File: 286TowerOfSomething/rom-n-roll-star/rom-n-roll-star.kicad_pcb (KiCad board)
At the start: 2 copper layers, 15 parts, among them J1 Bus_ISA_8bit, SW1 SW_DIP_x08, U1 SST39SF010, U2 74ALS688

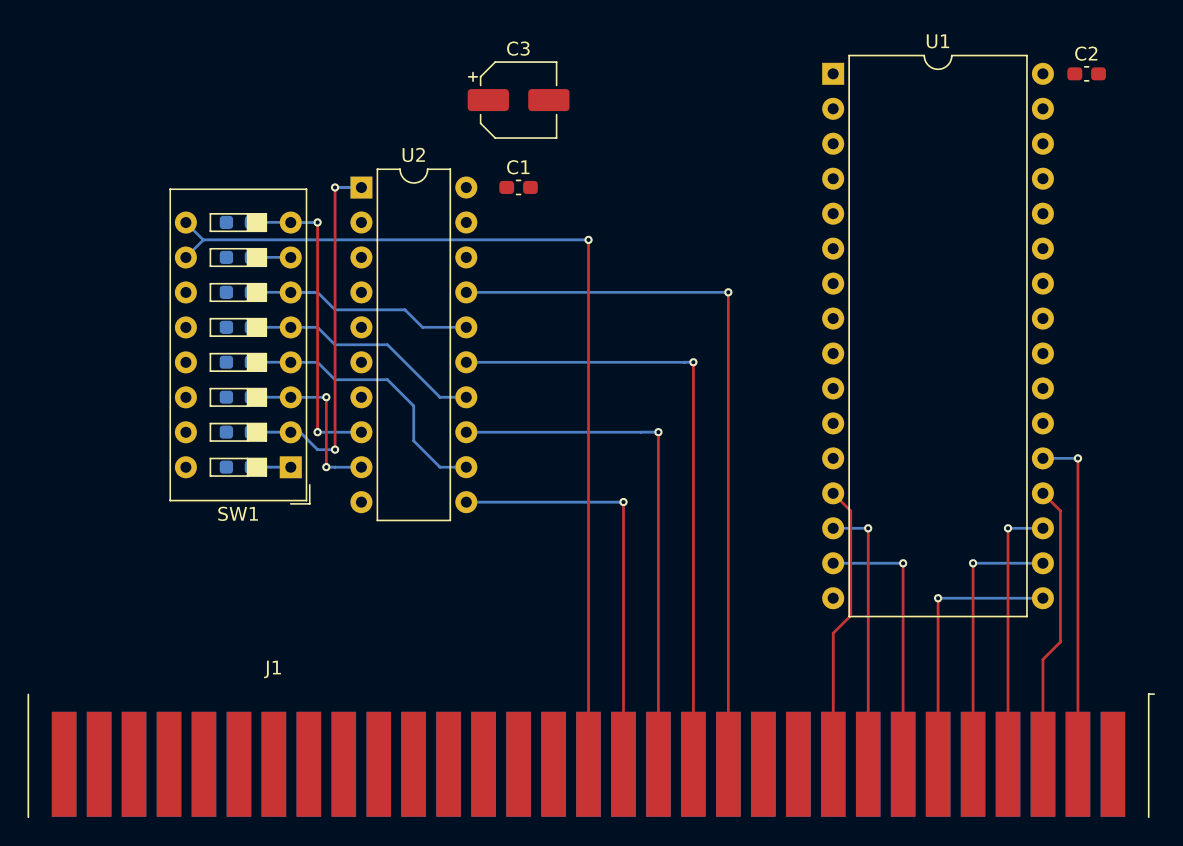
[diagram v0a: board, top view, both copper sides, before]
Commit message: Finished routing?
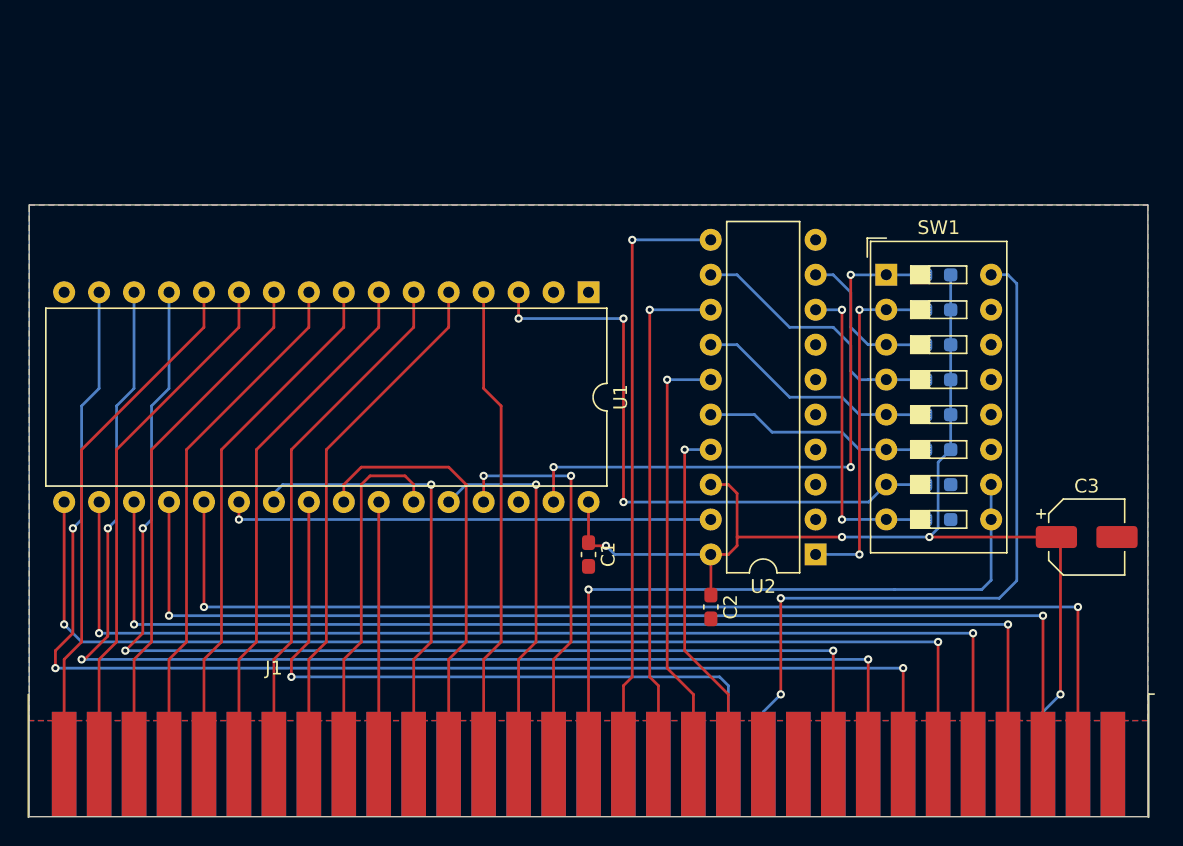
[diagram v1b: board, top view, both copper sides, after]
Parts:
- moved R1 55.2 mm to (139.7, 78.7), turned to 0 degrees
- moved R2 53.4 mm to (139.7, 76.2), turned to 180 degrees
- moved R3 52.7 mm to (139.7, 61.0), turned to 180 degrees
- moved C3 52.1 mm to (150.5, 80.0)
- moved R8 52.1 mm to (139.7, 73.7), turned to 180 degrees
- moved R4 51.6 mm to (139.7, 63.5), turned to 180 degrees
- moved R7 51.2 mm to (139.7, 71.1), turned to 180 degrees
- moved R5 50.9 mm to (139.7, 66.0), turned to 180 degrees
- moved R6 50.8 mm to (139.7, 68.6), turned to 180 degrees
- moved C2 47.4 mm to (123.2, 85.1), turned to -90 degrees
- moved SW1 45.5 mm to (135.9, 61.0), turned to 0 degrees
- moved U2 42.4 mm to (130.8, 81.3), turned to 180 degrees
- moved C1 27.1 mm to (114.3, 81.3), turned to -90 degrees
- moved U1 23.8 mm to (114.3, 62.2), turned to -90 degrees
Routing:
- net +5V: track 0.00 -> 83.4 mm, vias 0 -> 4
- net /D2: track 19.7 -> 97.2 mm, vias 1 -> 3
- net /D1: track 19.7 -> 93.1 mm, vias 1 -> 3
- net /D0: track 20.7 -> 87.0 mm, vias 0 -> 3
- net /D4: track 19.7 -> 82.6 mm, vias 1 -> 2
- net /D5: track 19.7 -> 82.6 mm, vias 1 -> 2
- net /D3: track 19.7 -> 81.8 mm, vias 1 -> 2
- net /D6: track 20.7 -> 82.6 mm, vias 0 -> 2
- net /D7: track 24.8 -> 82.6 mm, vias 1 -> 2
- net /~{MEMWR}: track 0.00 -> 54.0 mm, vias 0 -> 2
- net /~{MEMRD}: track 0.00 -> 51.0 mm, vias 0 -> 1
- net /FLASH_A15: track 2.86 -> 45.3 mm, vias 0 -> 3
- net /~{ROMWE}: track 2.86 -> 43.5 mm, vias 0 -> 3
- net /A3: track 0.00 -> 38.5 mm
- net /A1: track 0.00 -> 38.5 mm
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- added copper zone on B.Cu, net GND
- added copper zone on F.Cu, net GND
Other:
- board outline added: 81.3 x 44.4 mm
